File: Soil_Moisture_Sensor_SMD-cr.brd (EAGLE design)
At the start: 49.8 x 26.4 mm, 23 parts, among them IC1 ATMEGA328P

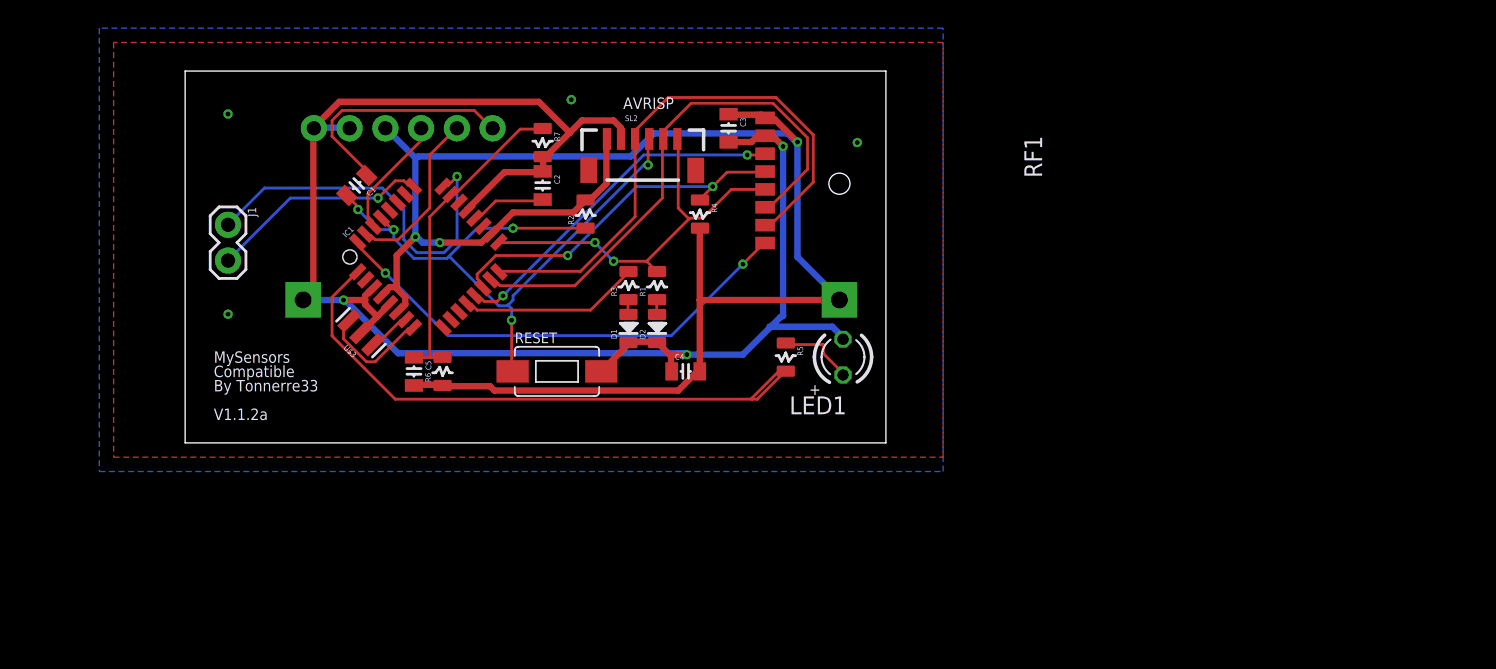
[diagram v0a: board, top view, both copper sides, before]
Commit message: 53x20
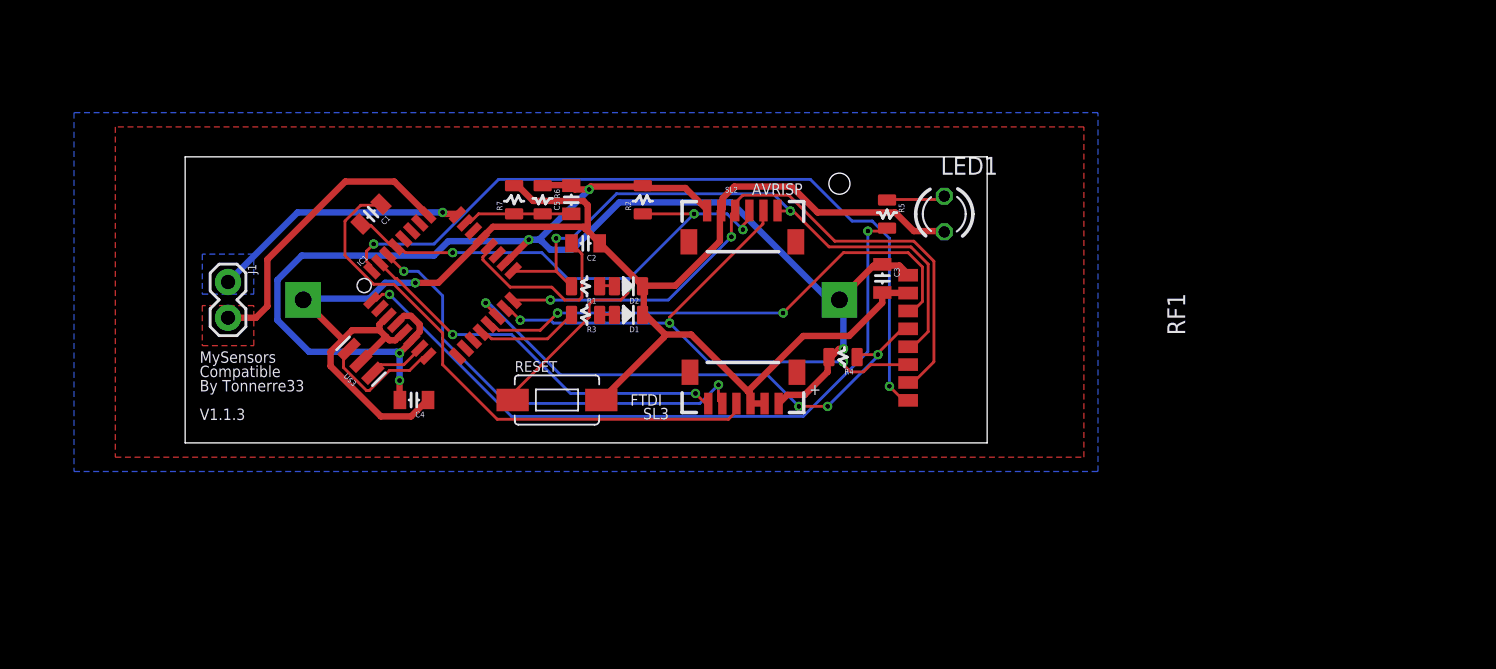
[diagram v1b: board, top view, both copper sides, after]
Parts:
- SL3: device SparkFun-Connectors:1X06 -> SparkFun-Connectors:1X06-1MM
- moved SL3 35.5 mm to (45.7, 14.2), flipped to the top
- moved C4 19.4 mm to (22.4, 13.2), turned to 180 degrees
- moved C5 16.5 mm to (33.5, 27.4), turned to 90 degrees
- moved C3 15.3 mm to (55.6, 21.8)
- moved RF1 15.1 mm to (67.1, 17.3)
- moved R4 14.4 mm to (52.8, 16.3), turned to 180 degrees
- moved R6 14.1 mm to (31.5, 27.4), turned to 270 degrees
- moved LED1 12.4 mm to (60.0, 26.4), turned to 270 degrees
- moved R5 12.4 mm to (56.0, 26.4)
- moved SL2 8.74 mm to (45.7, 25.4)
- moved C2 5.12 mm to (34.5, 24.3), turned to 180 degrees
- moved R1 5.08 mm to (34.5, 21.3), turned to 180 degrees
- moved R7 4.54 mm to (29.5, 27.4), turned to 90 degrees
- moved R2 4.19 mm to (38.6, 27.4)
- moved J1 4.06 mm to (9.14, 21.6)
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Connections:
- net D0_RX: now also SL3.5; no longer SL3.4
- net D1_TX: now also SL3.6; no longer SL3.5
- net DTR: now also SL3.4; no longer SL3.6
- net GND: now also SL3.3; no longer SL3.1
- net VCC: now also SL3.1; no longer SL3.3
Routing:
- net DTR: track 17.1 -> 40.3 mm
- net D0_RX: track 8.70 -> 31.7 mm, vias 0 -> 2
- net IRQ: track 34.5 -> 54.8 mm
- net VCC: track 122.3 -> 103.1 mm, vias 3 -> 5
- net SCK: track 28.7 -> 44.3 mm
- net D1_TX: track 12.1 -> 27.6 mm, vias 0 -> 2
- net A0: track 22.7 -> 7.80 mm
- net CSN: track 25.9 -> 38.4 mm, vias 2 -> 4
- net CE: track 25.1 -> 37.4 mm
- net N$5: track 26.7 -> 18.4 mm
- net N$4: track 5.37 -> 13.6 mm
- net N$9: track 43.4 -> 50.9 mm, vias 0 -> 2
- net MISO: track 40.2 -> 45.8 mm, vias 0 -> 2
- net N$6: track 12.8 -> 7.33 mm
- net N$3: track 15.7 -> 21.1 mm, vias 1 -> 0
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- added copper zone on layer 1, net N$3
- added copper zone on layer 16, net N$5
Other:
- board size 49.8 x 26.4 mm -> 57 x 20.3 mm
- board text added: "V1.1.3"
- board text removed: "DTR"
- board text removed: "GND"
- board text removed: "RX"
- board text removed: "TX"
- board text removed: "V1.1.2a"
- board text removed: "VCC"

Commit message: pcb-v1.1.3
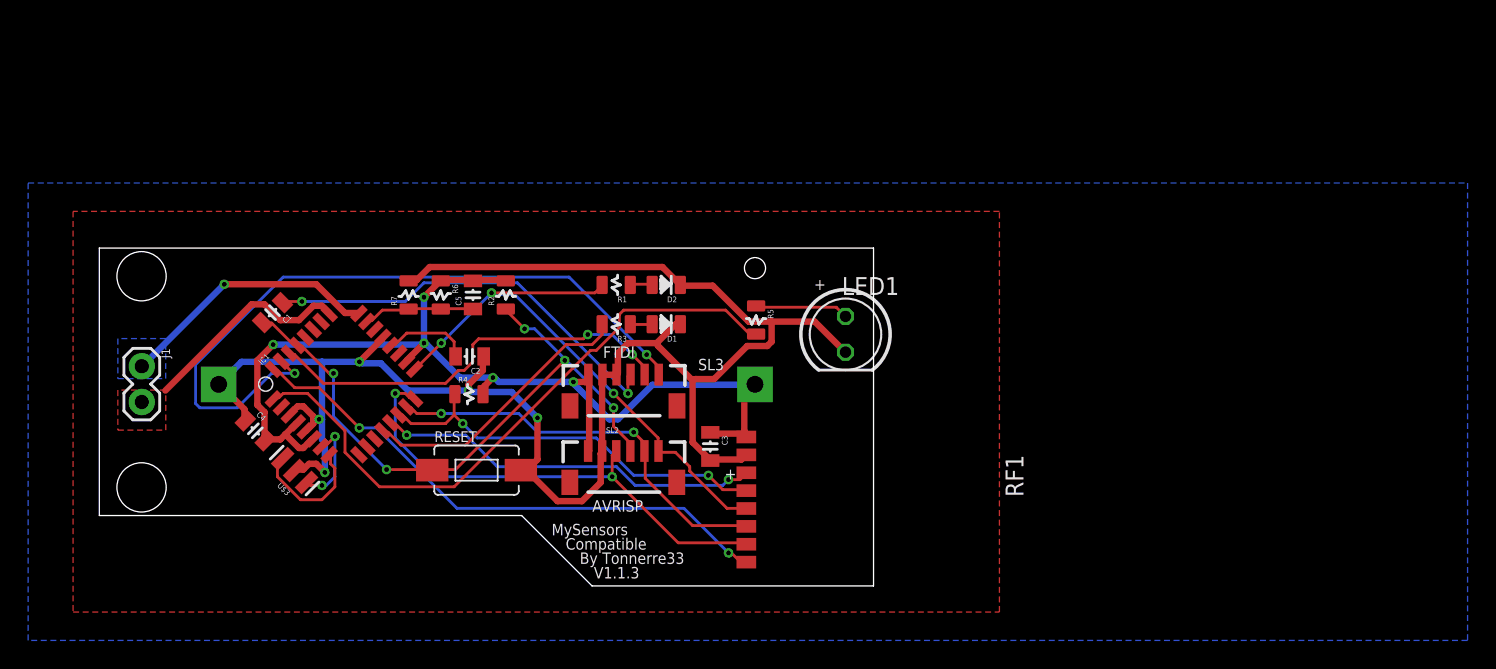
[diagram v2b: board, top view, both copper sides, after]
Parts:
- LED1: device led:LED3MM -> led:LED5MM
- moved R4 26.7 mm to (26.3, 13.6), turned to 0 degrees
- moved SL2 19.1 mm to (37.3, 8.31)
- moved C3 17.1 mm to (43.4, 9.91)
- moved RF1 16.3 mm to (55.6, 5.78)
- moved R5 12.0 mm to (46.7, 18.9)
- moved R2 11.8 mm to (28.9, 20.7)
- moved C2 11.5 mm to (26.3, 16.3)
- moved C4 11.5 mm to (11.1, 11.0), turned to 315 degrees
- moved LED1 11.1 mm to (53.0, 17.9)
- moved R7 10.1 mm to (22.0, 20.7)
- moved R6 9.91 mm to (24.3, 20.7)
- moved C1 9.90 mm to (12.3, 19.4)
- moved IC1 9.90 mm to (17.4, 14.3)
- moved C5 9.72 mm to (26.5, 20.7)
- moved U$3 9.08 mm to (13.9, 8.20)
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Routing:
- net VCC: track 103.1 -> 77.2 mm
- net D1_TX: track 27.6 -> 50.9 mm
- net IRQ: track 54.8 -> 39.3 mm
- net N$6: track 7.33 -> 20.0 mm
- net MOSI: track 41.6 -> 29.1 mm, vias 3 -> 2
- net MISO: track 45.8 -> 34.8 mm
- net DTR: track 40.3 -> 29.8 mm, vias 0 -> 2
- net CE: track 37.4 -> 27.5 mm
- net CSN: track 38.4 -> 28.9 mm, vias 4 -> 2
- net GND: track 122.1 -> 130.2 mm, vias 1 -> 5
- net N$4: track 13.6 -> 6.26 mm
- net N$9: track 50.9 -> 44.6 mm, vias 2 -> 0
- net N$3: track 21.1 -> 15.3 mm
- net RST: track 49.5 -> 45.1 mm, vias 4 -> 5
- net SCK: track 44.3 -> 41.1 mm, vias 2 -> 3
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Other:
- board size 57 x 20.3 mm -> 55 x 24 mm
